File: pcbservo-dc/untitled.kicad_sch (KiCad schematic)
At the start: 36 parts, among them IC1 NC7WZ241K8X, IC2 NC7WZ241K8X, IC3 NC7WZ241K8X, J7 Conn_ST_STDC14, J8 Conn_01x03, U7 STM32H573RITx

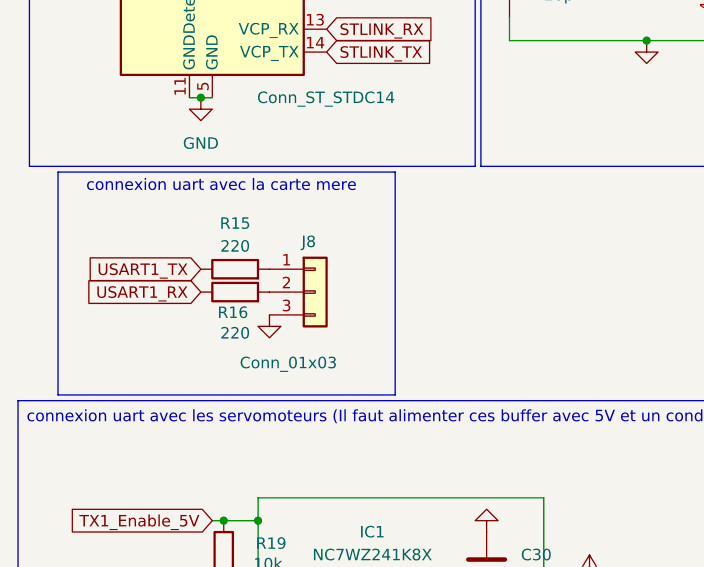
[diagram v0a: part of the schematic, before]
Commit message: uart a jour
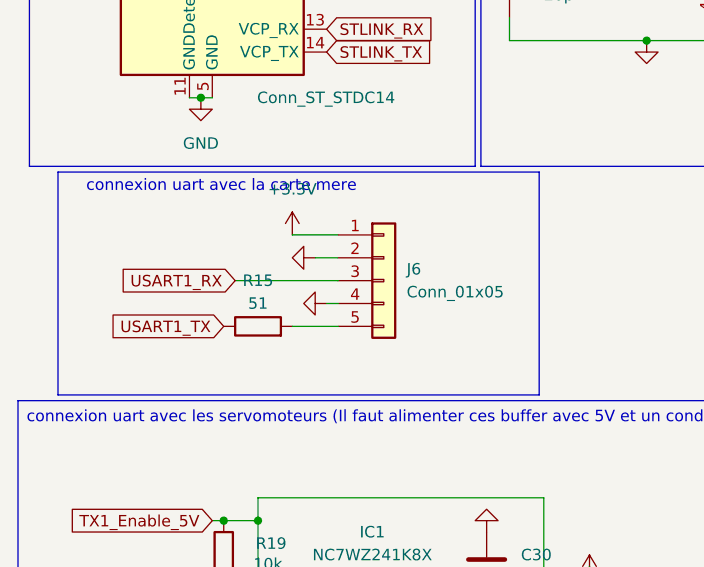
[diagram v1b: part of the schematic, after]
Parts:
- removed J8: Conn_01x03, Connector_JST:JST_PH_B3B-PH-K_1x03_P2.00mm_Vertical, symbol Connector_Generic:Conn_01x03
- removed R16: 220, Resistor_SMD:R_0402_1005Metric, symbol Device:R
- added J6: Conn_01x05, Connector_JST:JST_XH_B5B-XH-A_1x05_P2.50mm_Vertical, symbol Connector_Generic:Conn_01x05
- R15: value 220 -> 51
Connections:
- net +3.3V: now also J6.1 (Pin_1)
- net GND: now also J6.2 (Pin_2), J6.4 (Pin_4)
- net USART1_RX: now also J6.3 (Pin_3)
- net at R15.2: now also J6.5 (Pin_5)
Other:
- moved on the sheet: R15

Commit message: changement de quelques empreinte
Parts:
- J6: footprint Connector_JST:JST_XH_B5B-XH-A_1x05_P2.50mm_Vertical -> Connector_JST:JST_EH_B5B-EH-A_1x05_P2.50mm_Vertical
